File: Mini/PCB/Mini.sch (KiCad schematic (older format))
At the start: 30 parts

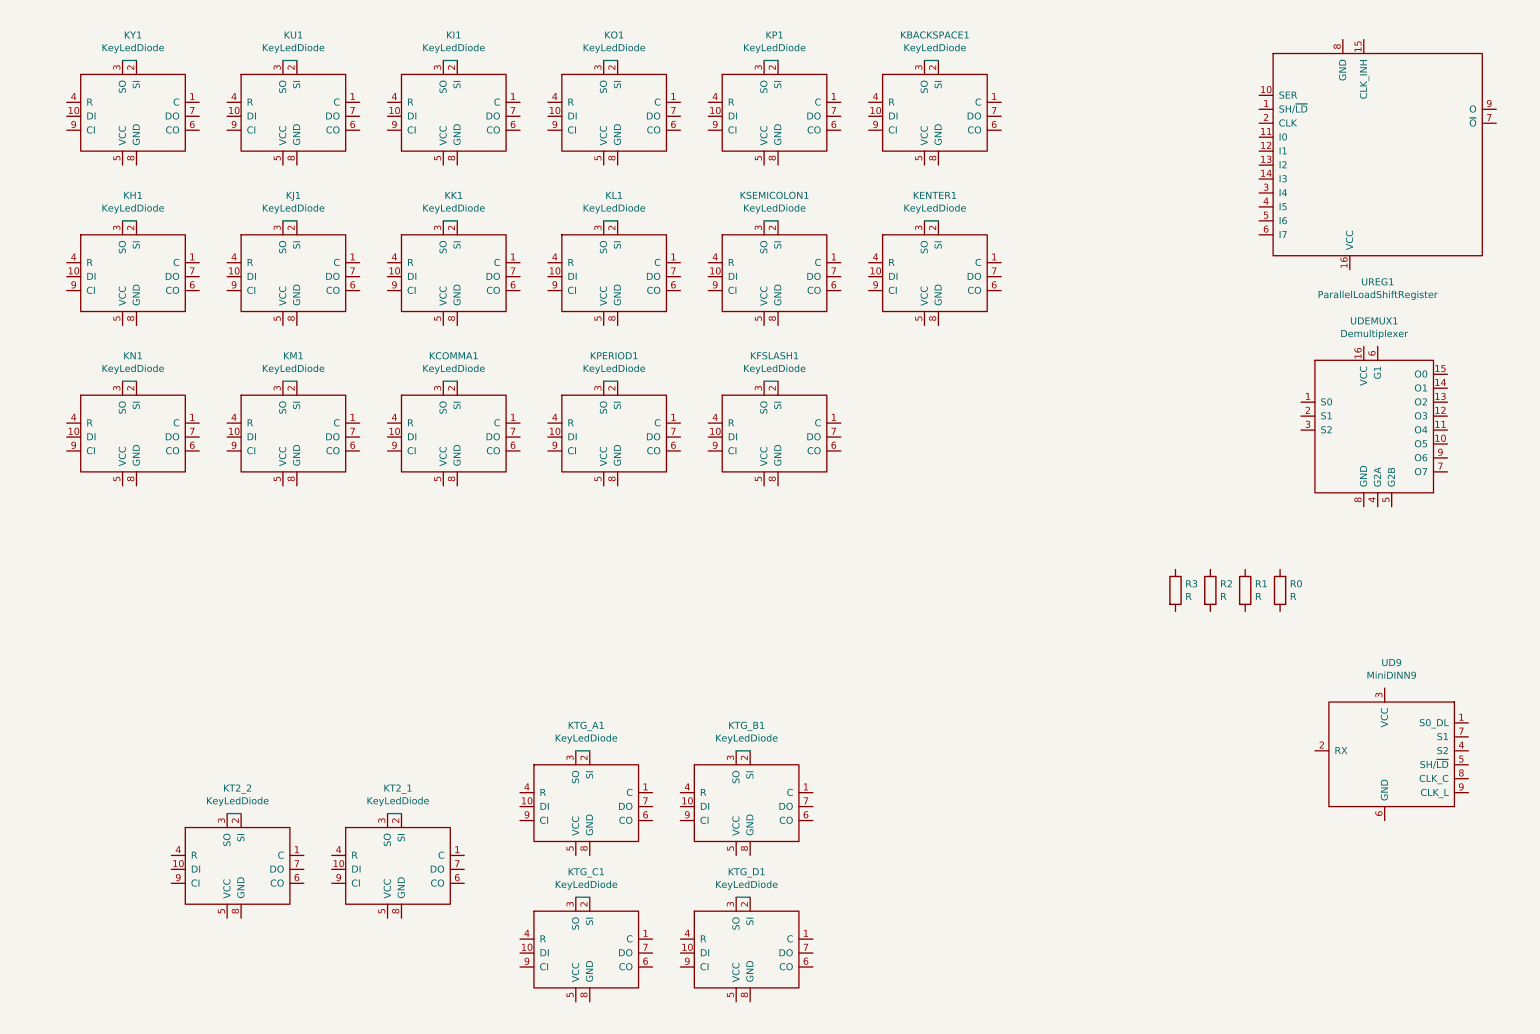
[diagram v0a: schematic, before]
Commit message: Wiring up all pins on schematic.
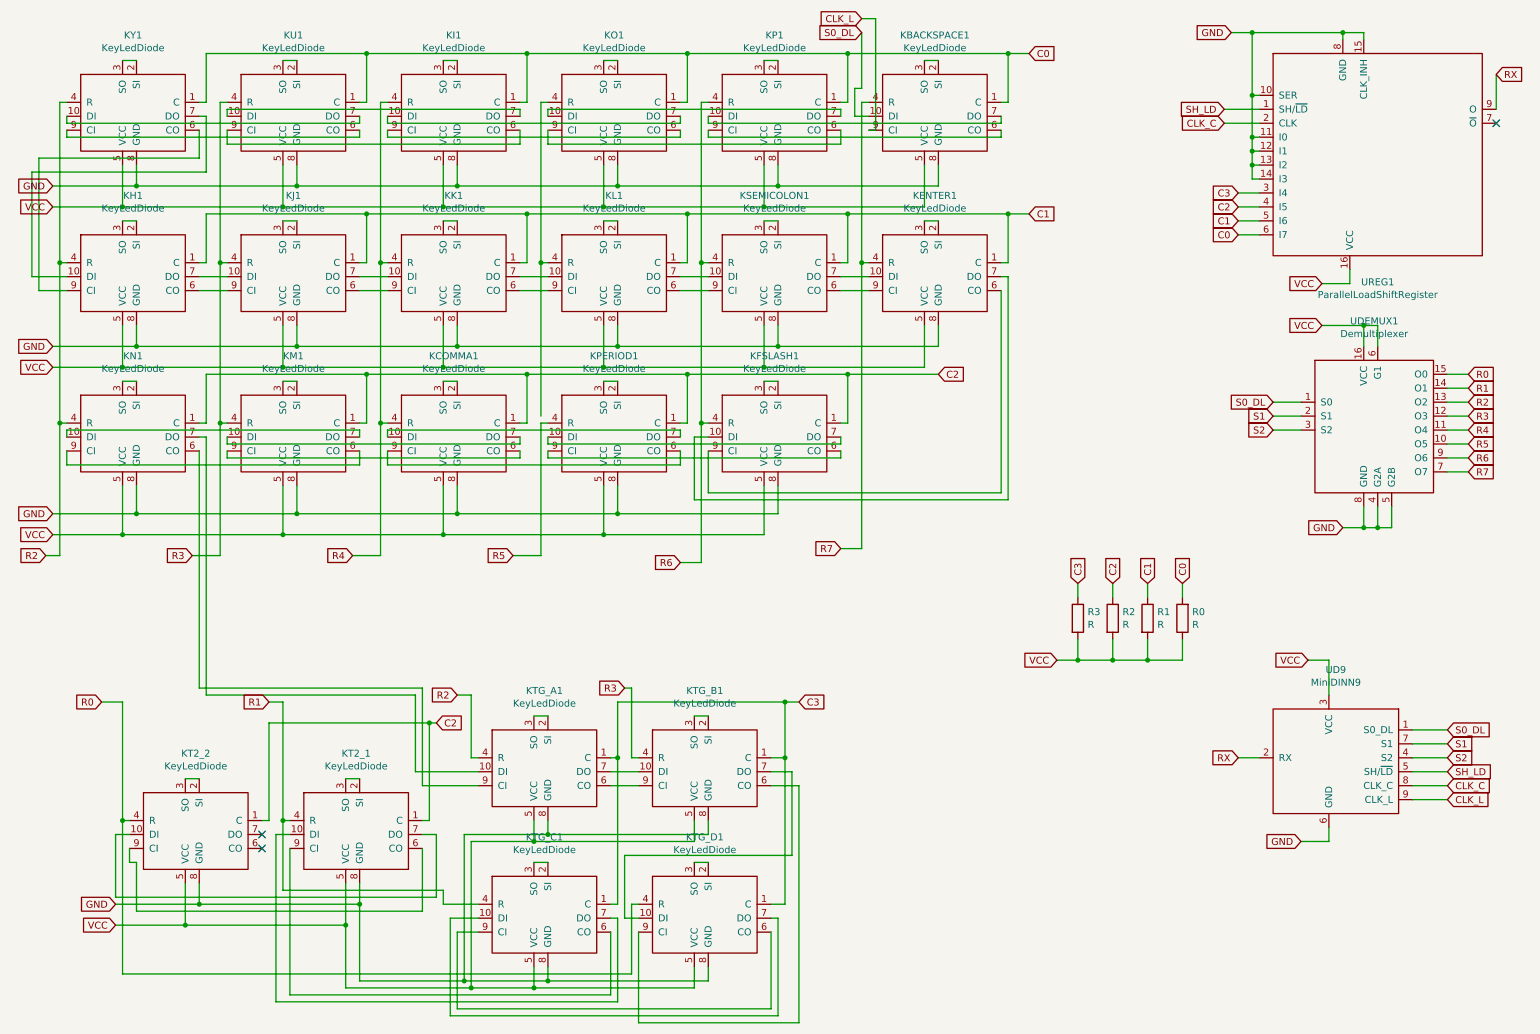
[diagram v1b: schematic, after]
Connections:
- net S0_DL: now reaches UD9.1 (S0_DL)
- net S0_DL: now also KBACKSPACE1.10 (DI), UDEMUX1.1 (S0)
- net RX: now reaches UD9.2 (RX)
- net RX: now also UREG1.9 (O)
- net VCC: now reaches UD9.3 (VCC)
- net VCC: now also KBACKSPACE1.5 (VCC), KCOMMA1.5 (VCC), KENTER1.5 (VCC), KFSLASH1.5 (VCC), KH1.5 (VCC), KI1.5 (VCC), KJ1.5 (VCC), KK1.5 (VCC), KL1.5 (VCC), KM1.5 (VCC), KN1.5 (VCC), KO1.5 (VCC), KP1.5 (VCC), KPERIOD1.5 (VCC), KSEMICOLON1.5 (VCC), KT2_1.5 (VCC), KT2_2.5 (VCC), KTG_A1.5 (VCC), KTG_B1.5 (VCC), KTG_C1.5 (VCC), KTG_D1.5 (VCC), KU1.5 (VCC), KY1.5 (VCC), R0.1, R1.2, R2.2, R3.2, UDEMUX1.16 (VCC), UDEMUX1.6 (G1), UREG1.16 (VCC)
- net S2: now reaches UD9.4 (S2)
- net S2: now also UDEMUX1.3 (S2)
- net SH_LD: now reaches UD9.5 (SH/~LD)
- net SH_LD: now also UREG1.1 (SH/~LD)
- net GND: now reaches UD9.6 (GND)
- net GND: now also KBACKSPACE1.8 (GND), KCOMMA1.8 (GND), KENTER1.8 (GND), KFSLASH1.8 (GND), KH1.8 (GND), KI1.8 (GND), KJ1.8 (GND), KK1.8 (GND), KL1.8 (GND), KM1.8 (GND), KN1.8 (GND), KO1.8 (GND), KP1.8 (GND), KPERIOD1.8 (GND), KSEMICOLON1.8 (GND), KT2_1.8 (GND), KT2_2.8 (GND), KTG_A1.8 (GND), KTG_B1.8 (GND), KTG_C1.8 (GND), KTG_D1.8 (GND), KU1.8 (GND), KY1.8 (GND), UDEMUX1.4 (G2A), UDEMUX1.5 (G2B), UDEMUX1.8 (GND), UREG1.10 (SER), UREG1.11 (I0), UREG1.12 (I1), UREG1.13 (I2), UREG1.14 (I3), UREG1.15 (CLK_INH), UREG1.8 (GND)
- net S1: now reaches UD9.7 (S1)
- net S1: now also UDEMUX1.2 (S1)
- net CLK_C: now reaches UD9.8 (CLK_C)
- net CLK_C: now also UREG1.2 (CLK)
- net CLK_L: now reaches UD9.9 (CLK_L)
- net CLK_L: now also KBACKSPACE1.9 (CI)
- net R5: now reaches UDEMUX1.10 (O5)
- net R5: now also KPERIOD1.4 (R)
- net R4: now reaches UDEMUX1.11 (O4)
- net R4: now also KCOMMA1.4 (R), KI1.4 (R), KK1.4 (R)
- net R3: now reaches UDEMUX1.12 (O3)
- net R3: now also KJ1.4 (R), KM1.4 (R), KTG_B1.4 (R), KU1.4 (R)
- net R2: now reaches UDEMUX1.13 (O2)
- net R2: now also KH1.4 (R), KN1.4 (R), KTG_A1.4 (R), KY1.4 (R)
- net R1: now reaches UDEMUX1.14 (O1)
- net R1: now also KT2_1.4 (R), KTG_C1.4 (R)
- net R0: now reaches UDEMUX1.15 (O0)
- net R0: now also KT2_2.4 (R), KTG_D1.4 (R)
- net R7: now reaches UDEMUX1.7 (O7)
- net R7: now also KBACKSPACE1.4 (R), KENTER1.4 (R)
- net R6: now reaches UDEMUX1.9 (O6)
- net R6: now also KFSLASH1.4 (R), KP1.4 (R), KSEMICOLON1.4 (R)
- net C3: now reaches UREG1.3 (I4)
- net C3: now also KTG_A1.1 (C), KTG_B1.1 (C), KTG_C1.1 (C), KTG_D1.1 (C), R3.1
- net C2: now reaches UREG1.4 (I5)
- net C2: now also KCOMMA1.1 (C), KFSLASH1.1 (C), KM1.1 (C), KN1.1 (C), KPERIOD1.1 (C), KT2_1.1 (C), KT2_2.1 (C), R2.1
- net C1: now reaches UREG1.5 (I6)
- net C1: now also KENTER1.1 (C), KH1.1 (C), KJ1.1 (C), KK1.1 (C), KL1.1 (C), KSEMICOLON1.1 (C), R1.1
- net C0: now reaches UREG1.6 (I7)
- net C0: now also KBACKSPACE1.1 (C), KI1.1 (C), KO1.1 (C), KP1.1 (C), KU1.1 (C), KY1.1 (C), R0.2
- net at KY1.10 (DI): now also KU1.7 (DO)
- net at KY1.6 (CO): now also KH1.9 (CI)
- net at KY1.7 (DO): now also KH1.10 (DI)
- net at KY1.9 (CI): now also KU1.6 (CO)
- net at KU1.10 (DI): now also KI1.7 (DO)
- net at KU1.9 (CI): now also KI1.6 (CO)
- net at KI1.10 (DI): now also KO1.7 (DO)
- net at KI1.9 (CI): now also KO1.6 (CO)
- net at KO1.10 (DI): now also KP1.7 (DO)
- net at KO1.4 (R): now also KL1.4 (R)
- net at KO1.9 (CI): now also KP1.6 (CO)
- net at KP1.10 (DI): now also KBACKSPACE1.7 (DO)
- net at KP1.9 (CI): now also KBACKSPACE1.6 (CO)
- net at KENTER1.10 (DI): now also KSEMICOLON1.7 (DO)
- net at KENTER1.6 (CO): now also KFSLASH1.9 (CI)
- net at KENTER1.7 (DO): now also KFSLASH1.10 (DI)
- net at KENTER1.9 (CI): now also KSEMICOLON1.6 (CO)
- net at KH1.6 (CO): now also KJ1.9 (CI)
- net at KH1.7 (DO): now also KJ1.10 (DI)
- net at KN1.10 (DI): now also KM1.7 (DO)
- net at KN1.6 (CO): now also KTG_A1.9 (CI)
- net at KN1.7 (DO): now also KTG_A1.10 (DI)
- net at KN1.9 (CI): now also KM1.6 (CO)
- net at KJ1.6 (CO): now also KK1.9 (CI)
- net at KJ1.7 (DO): now also KK1.10 (DI)
- net at KM1.10 (DI): now also KCOMMA1.7 (DO)
- net at KM1.9 (CI): now also KCOMMA1.6 (CO)
- net at KK1.6 (CO): now also KL1.9 (CI)
- net at KK1.7 (DO): now also KL1.10 (DI)
- net at KCOMMA1.10 (DI): now also KPERIOD1.7 (DO)
- net at KCOMMA1.9 (CI): now also KPERIOD1.6 (CO)
- net at KL1.6 (CO): now also KSEMICOLON1.9 (CI)
- net at KL1.7 (DO): now also KSEMICOLON1.10 (DI)
- net at KPERIOD1.10 (DI): now also KFSLASH1.7 (DO)
- net at KPERIOD1.9 (CI): now also KFSLASH1.6 (CO)
- net at KT2_1.10 (DI): now also KTG_C1.7 (DO)
- net at KT2_1.6 (CO): now also KT2_2.9 (CI)
- net at KT2_1.7 (DO): now also KT2_2.10 (DI)
- net at KT2_1.9 (CI): now also KTG_C1.6 (CO)
- net at KTG_A1.6 (CO): now also KTG_B1.9 (CI)
- net at KTG_A1.7 (DO): now also KTG_B1.10 (DI)
- net at KTG_B1.6 (CO): now also KTG_D1.9 (CI)
- net at KTG_B1.7 (DO): now also KTG_D1.10 (DI)
- net at KTG_C1.10 (DI): now also KTG_D1.7 (DO)
- net at KTG_C1.9 (CI): now also KTG_D1.6 (CO)
- no-connect marks 0 -> 3
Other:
- moved on the sheet: KT2_1, KT2_2, KTG_A1, KTG_B1, KTG_C1, KTG_D1, R0, R1, R2, R3, UD9
